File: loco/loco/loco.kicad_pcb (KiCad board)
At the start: 2 copper layers, 19.3 x 11.3 mm, 33 parts, among them Q1 FDC6561AN, Q2 FDC6561AN, Q3 FDC6561AN, U1 STM32F030F4Px, U2 A4953_LJ, U3 TLV760

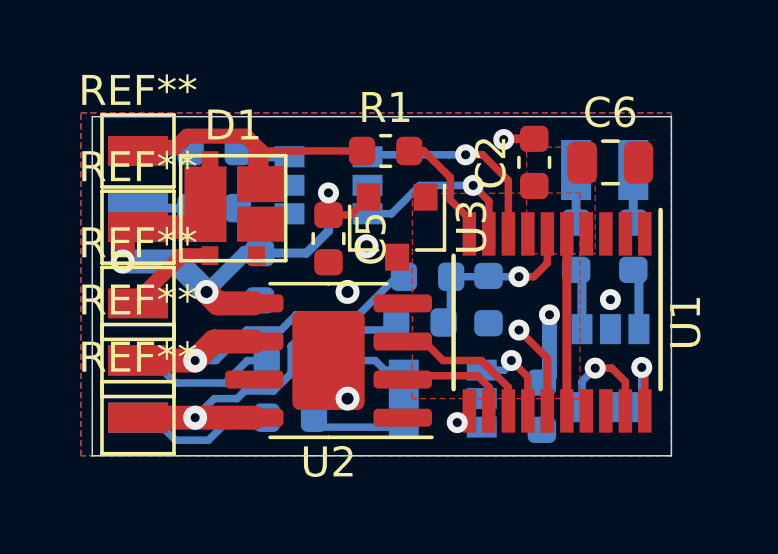
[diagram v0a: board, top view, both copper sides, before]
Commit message: PCB update
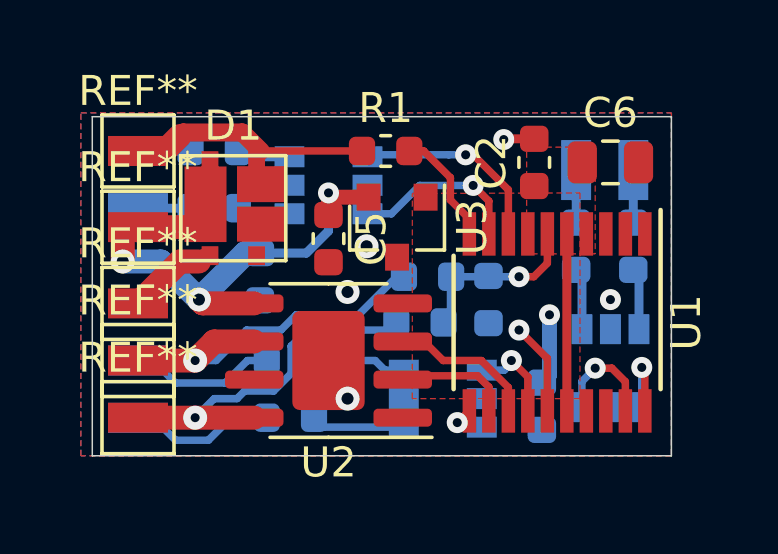
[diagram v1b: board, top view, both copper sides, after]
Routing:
- net RAIL1: track 9.73 -> 8.73 mm
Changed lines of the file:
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@@
   )
   (setup
-    (last_trace_width 0.25)
+    (last_trace_width 0.5)
     (user_trace_width 0.3)
     (user_trace_width 0.5)
@@
   (segment (start 119.5225 81.6025) (end 119.67 81.75) (width 0.25) (layer F.Cu) (net 6))
   (segment (start 119.5225 80.965) (end 119.5225 81.6025) (width 0.25) (layer F.Cu) (net 6))
-  (segment (start 119.67 80.65) (end 119.67 81.75) (width 0.5) (layer F.Cu) (net 6))
-  (segment (start 119.17 80.15) (end 119.67 80.65) (width 0.5) (layer F.Cu) (net 6))
-  (segment (start 117.208 80.15) (end 119.17 80.15) (width 0.5) (layer F.Cu) (net 6))
-  (segment (start 116.84 80.518) (end 117.208 80.15) (width 0.5) (layer F.Cu) (net 6))
-  (segment (start 115.57 80.645) (end 115.697 80.518) (width 0.5) (layer F.Cu) (net 6))
-  (segment (start 115.697 80.518) (end 116.84 80.518) (width 0.5) (layer F.Cu) (net 6))
+  (segment (start 116.586 80.518) (end 116.954 80.15) (width 0.8) (layer F.Cu) (net 6))
+  (segment (start 119.04701 80.02701) (end 119.67 80.65) (width 0.6) (layer F.Cu) (net 6))
+  (segment (start 116.954 80.15) (end 117.07699 80.02701) (width 0.6) (layer F.Cu) (net 6))
+  (segment (start 117.07699 80.02701) (end 119.04701 80.02701) (width 0.6) (layer F.Cu) (net 6))
+  (segment (start 115.697 80.518) (end 115.57 80.645) (width 0.5) (layer F.Cu) (net 6))
+  (segment (start 116.586 80.518) (end 115.697 80.518) (width 0.5) (layer F.Cu) (net 6))
   (via (at 115.062 84.328) (size 0.8) (drill 0.4) (layers F.Cu B.Cu) (net 7))
-  (via (at 117.856 85.344) (size 0.8) (drill 0.4) (layers F.Cu B.Cu) (net 7))
-  (segment (start 122.6625 82.7785) (end 123.256 82.185) (width 0.25) (layer F.Cu) (net 7))
-  (segment (start 121.92 82.7785) (end 122.6625 82.7785) (width 0.25) (layer F.Cu) (net 7))
   (via (at 121.92 82.042) (size 0.7) (drill 0.3) (layers F.Cu B.Cu) (net 7))
   (segment (start 121.92 82.7785) (end 121.92 82.042) (width 0.5) (layer F.Cu) (net 7))
   (segment (start 117.97 82.27) (end 117.82 82.42) (width 0.25) (layer F.Cu) (net 7))
   (segment (start 117.97 80.965) (end 117.97 82.27) (width 0.25) (layer F.Cu) (net 7))
-  (segment (start 118.237 85.725) (end 117.856 85.344) (width 0.8) (layer F.Cu) (net 7))
-  (segment (start 119.445 85.725) (end 118.237 85.725) (width 0.8) (layer F.Cu) (net 7))
   (segment (start 117.055 83.185) (end 117.82 82.42) (width 0.5) (layer F.Cu) (net 7))
   (segment (start 115.57 83.185) (end 117.055 83.185) (width 0.8) (layer F.Cu) (net 7))
@@
   (segment (start 121.92 82.042) (end 121.92 83.312) (width 0.3) (layer B.Cu) (net 7))
   (segment (start 121.92 83.312) (end 121.1835 84.0485) (width 0.3) (layer B.Cu) (net 7))
-  (segment (start 119.1515 84.0485) (end 117.856 85.344) (width 0.5) (layer B.Cu) (net 7))
-  (segment (start 119.634 84.0485) (end 119.1515 84.0485) (width 0.5) (layer B.Cu) (net 7))
-  (segment (start 116.84 84.328) (end 117.856 85.344) (width 0.8) (layer B.Cu) (net 7))
-  (segment (start 115.062 84.328) (end 116.84 84.328) (width 0.8) (layer B.Cu) (net 7))
-  (segment (start 117.033 84.135) (end 117.97 84.135) (width 0.5) (layer F.Cu) (net 8))
-  (segment (start 115.57 85.725) (end 115.57 85.598) (width 0.5) (layer F.Cu) (net 8))
-  (segment (start 115.57 85.598) (end 117.033 84.135) (width 0.5) (layer F.Cu) (net 8))
+  (segment (start 122.063 82.185) (end 121.92 82.042) (width 0.5) (layer F.Cu) (net 7))
+  (segment (start 123.256 82.185) (end 122.063 82.185) (width 0.5) (layer F.Cu) (net 7))
+  (segment (start 116.331996 84.328) (end 117.601996 85.598) (width 0.8) (layer B.Cu) (net 7))
+  (segment (start 119.151496 84.0485) (end 117.601996 85.598) (width 0.8) (layer B.Cu) (net 7))
+  (segment (start 117.728996 85.725) (end 117.601996 85.598) (width 0.8) (layer F.Cu) (net 7))
+  (via (at 117.601996 85.598) (size 0.8) (drill 0.4) (layers F.Cu B.Cu) (net 7))
+  (segment (start 115.062 84.328) (end 116.331996 84.328) (width 0.8) (layer B.Cu) (net 7))
+  (segment (start 119.445 85.725) (end 117.728996 85.725) (width 0.8) (layer F.Cu) (net 7))
+  (segment (start 119.634 84.0485) (end 119.151496 84.0485) (width 0.8) (layer B.Cu) (net 7))
+  (segment (start 117.97 84.135) (end 117.795 84.135) (width 0.5) (layer F.Cu) (net 8))
+  (segment (start 116.967 84.328) (end 115.57 85.725) (width 0.8) (layer F.Cu) (net 8))
+  (segment (start 117.602 84.328) (end 116.967 84.328) (width 0.8) (layer F.Cu) (net 8))
   (via (at 129.286 86.106) (size 0.7) (drill 0.3) (layers F.Cu B.Cu) (net 9))
   (segment (start 124.841 85.725) (end 124.395 85.725) (width 0.25) (layer F.Cu) (net 9))
@@
   (segment (start 123.22 82.738) (end 124.018 82.738) (width 0.25) (layer B.Cu) (net 35))
   (segment (start 124.018 82.738) (end 124.96334 81.79266) (width 0.25) (layer B.Cu) (net 35))
-  (segment (start 127.915 81.629315) (end 127.057685 80.772) (width 0.25) (layer F.Cu) (net 36))
   (segment (start 123.19 80.772) (end 125.926315 80.772) (width 0.25) (layer B.Cu) (net 36))
-  (segment (start 127.057685 80.772) (end 126.492 80.772) (width 0.25) (layer F.Cu) (net 36))
   (segment (start 125.926315 80.772) (end 126.492 80.772) (width 0.25) (layer B.Cu) (net 36))
   (via (at 126.492 80.772) (size 0.7) (drill 0.3) (layers F.Cu B.Cu) (net 36))
-  (segment (start 127.915 83.41) (end 127.915 81.629315) (width 0.25) (layer F.Cu) (net 36))
+  (segment (start 126.746 80.772) (end 126.492 80.772) (width 0.25) (layer F.Cu) (net 36))
+  (segment (start 127.915 83.41) (end 127.915 81.941) (width 0.25) (layer F.Cu) (net 36))
+  (segment (start 127.915 81.941) (end 126.746 80.772) (width 0.25) (layer F.Cu) (net 36))
   (zone (net 5) (net_name GND) (layer F.Cu) (hatch full 0.508)
     (connect_pads yes (clearance 0.254))
